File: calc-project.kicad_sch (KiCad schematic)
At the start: 39 parts, among them J1 PinSocket_1x20_Right, J2 PinSocket_1x20_Left, J3 Conn_01x14, SW1 SW_Push_45deg, SW10 SW_Push_45deg, SW11 SW_Push_45deg, SW12 SW_Push_45deg, SW13 SW_Push_45deg, SW14 SW_Push_45deg, SW15 SW_Push_45deg, SW16 SW_Push_45deg, SW17 SW_Push_45deg, SW18 SW_Push_45deg, SW19 SW_Push_45deg, SW2 SW_Push_45deg, SW20 SW_Push_45deg, SW21 SW_Push_45deg, SW22 SW_Push_45deg, SW23 SW_Push_45deg, SW24 SW_Push_45deg, SW25 SW_Push_45deg, SW26 SW_Push_45deg, SW27 SW_Push_45deg, SW28 SW_Push_45deg, SW29 SW_Push_45deg, SW3 SW_Push_45deg, SW30 SW_Push_45deg, SW31 SW_Push_45deg, SW32 SW_Push_45deg, SW33 SW_Push_45deg, SW34 SW_Push_45deg, SW35 SW_Push_45deg, SW36 SW_Push_45deg, SW4 SW_Push_45deg, SW5 SW_Push_45deg, SW6 SW_Push_45deg, SW7 SW_Push_45deg, SW8 SW_Push_45deg, SW9 SW_Push_45deg

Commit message: capabilities
yeah
did use kicad happy just to check and make sure we had capabilities
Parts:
- J1, J2: KiLib_Generator (none) -> connector/pin_header_socket
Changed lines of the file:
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@@
+			)
+		)
+		(property "KiLib_Generator" "connector/pin_header_socket"
+			(at 173.99 45.72 0)
+			(hide yes)
+			(show_name no)
+			(do_not_autoplace no)
+			(effects
+				(font
+					(size 1.27 1.27)
+				)
 			)
 		)
@@
 			(at 231.14 45.72 0)
 			(hide yes)
+			(show_name no)
+			(do_not_autoplace no)
+			(effects
+				(font
+					(size 1.27 1.27)
+				)
+			)
+		)
+		(property "KiLib_Generator" "connector/pin_header_socket"
+			(at 231.14 45.72 0)
+			(hide yes)

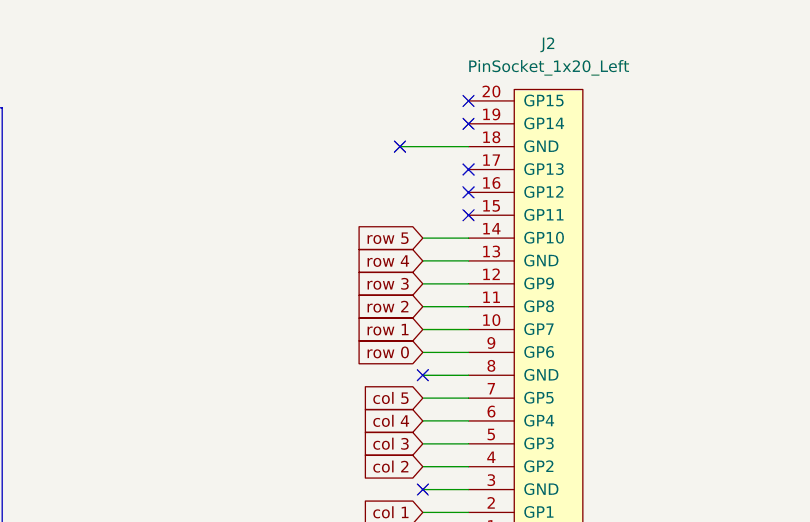
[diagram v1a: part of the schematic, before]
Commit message: wrong pin
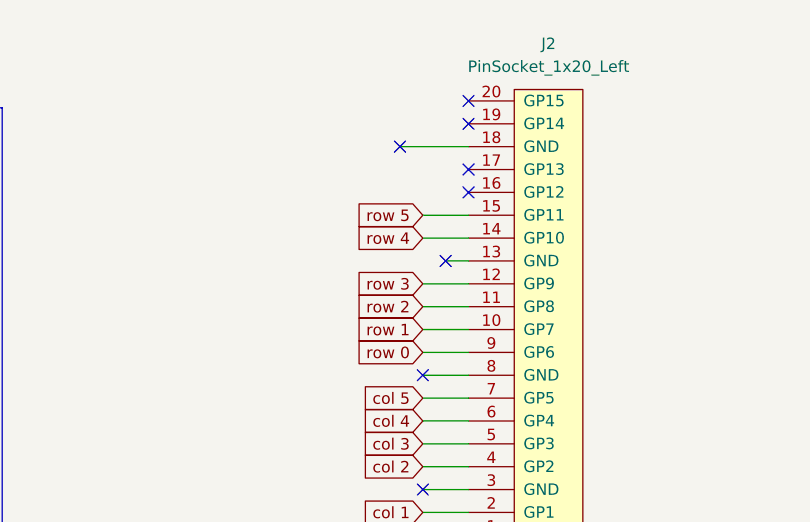
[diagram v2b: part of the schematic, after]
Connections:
- net row 4: now also J2.14 (GP10); no longer J2.13 (GND)
- net row 5: now also J2.15 (GP11); no longer J2.14 (GP10)
